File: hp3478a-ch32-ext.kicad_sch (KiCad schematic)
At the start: 50 parts, among them J1 Conn_GPIB, J2 Pwr, J4 USB, J5 Micro_SD_Card_Det1, J6 DEBUG, Q1 BSS138, SW1 RST, U1 CH32V203CxTx, U2 TLV76701DRVx, U3 AHT20, Y1 24MHz, 10pF

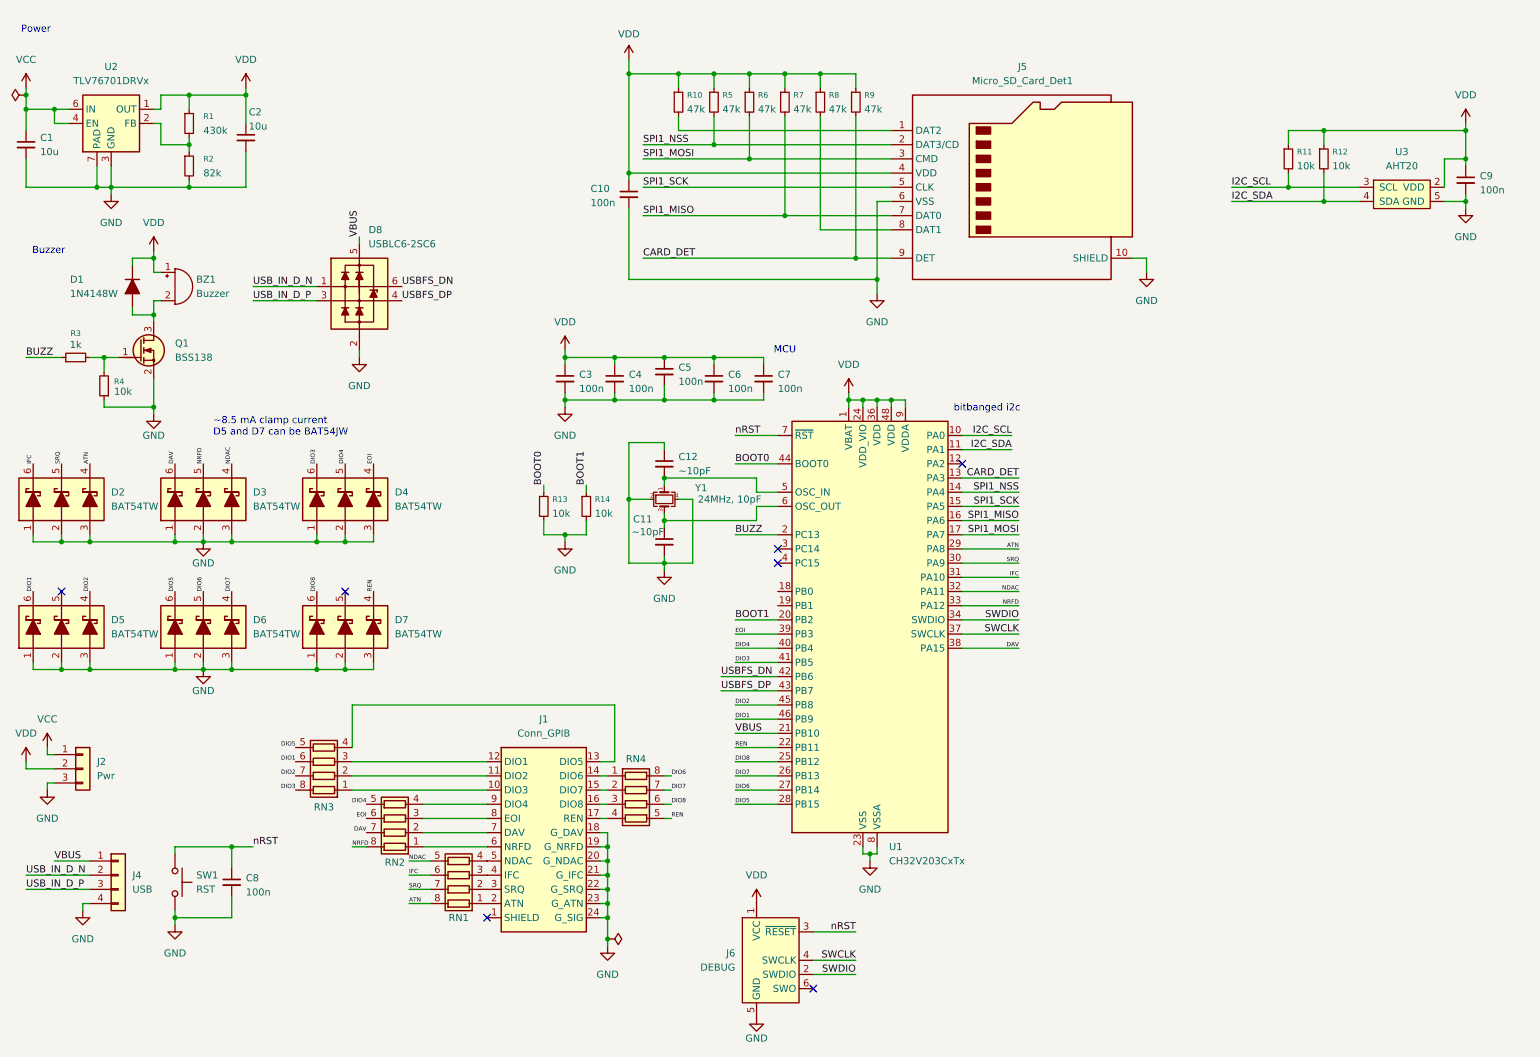
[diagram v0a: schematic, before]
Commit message: chore: upd
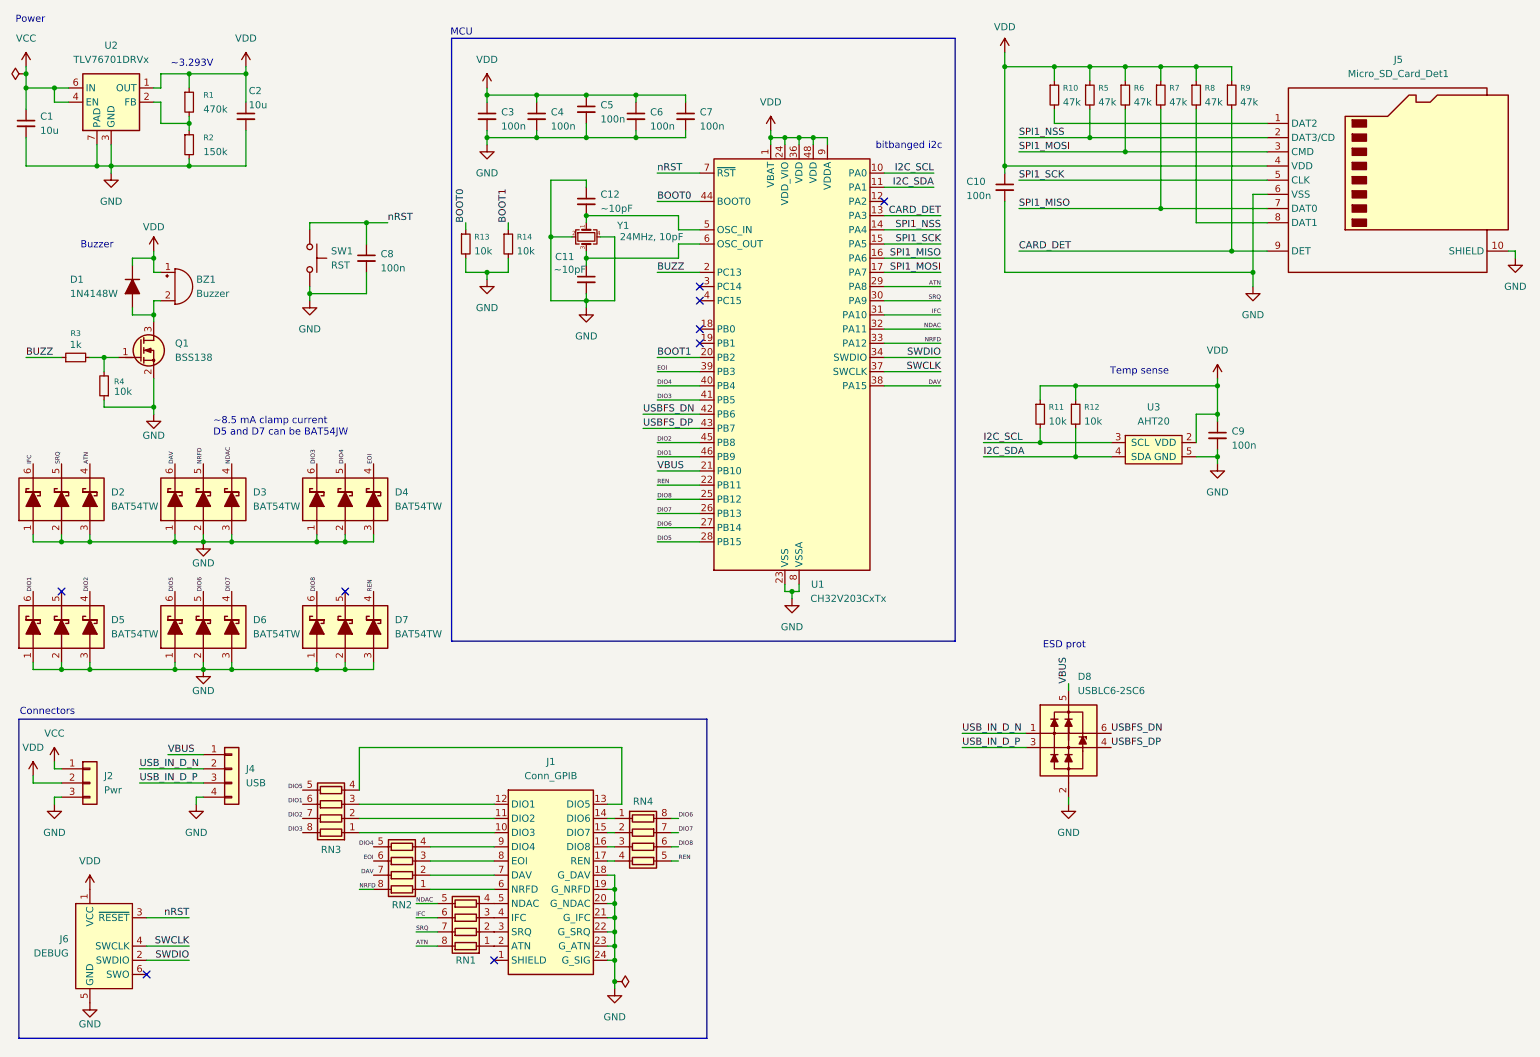
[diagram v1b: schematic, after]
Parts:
- R1: value 430k -> 470k
- R2: value 82k -> 150k
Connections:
- no-connect marks 7 -> 9
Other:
- note added: "Connectors"
- note added: "ESD prot"
- note added: "Temp sense"
- note added: "~3.293V"
- company: (none) -> kuwoyuki
- title: (none) -> HP3478A Extension
- moved on the sheet: C1, C10, C11, C12, C2, C3, C4, C5, C6, C7, C8, C9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
